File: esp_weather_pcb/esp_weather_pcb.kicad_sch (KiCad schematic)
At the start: 6 parts, among them U1 esp32_38P_Left, U2 esp32_38P_Right

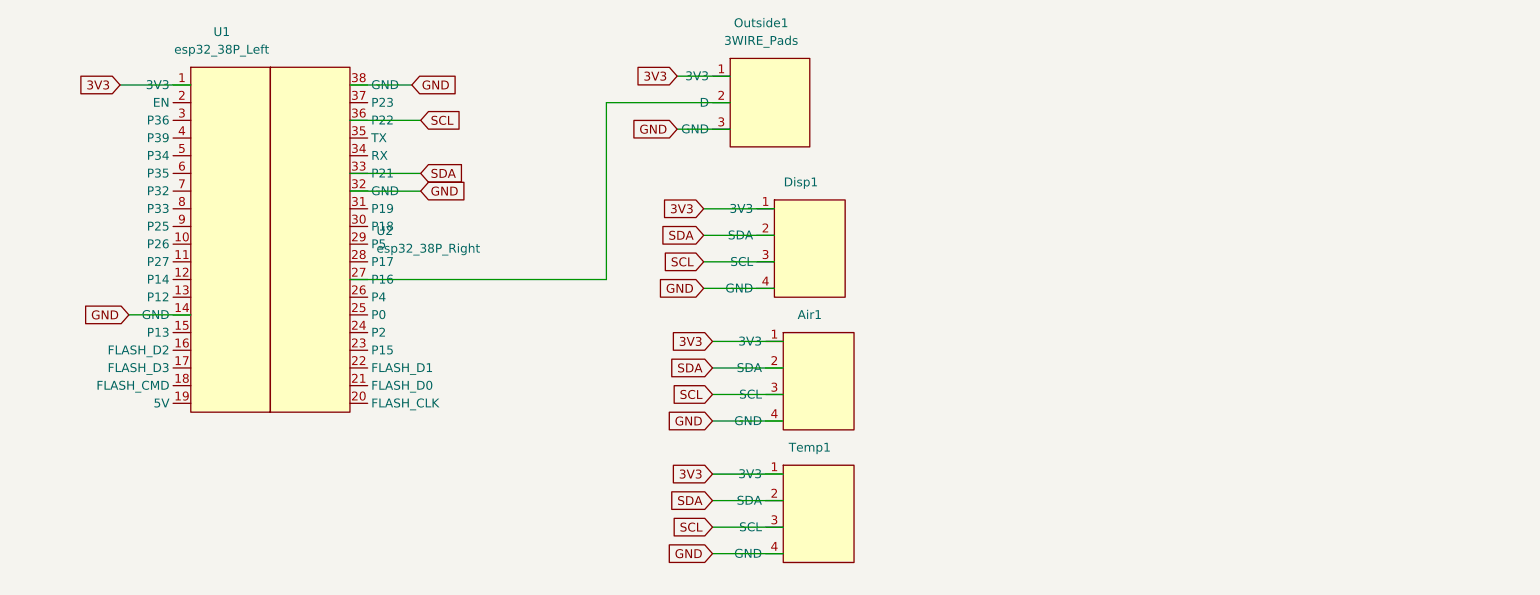
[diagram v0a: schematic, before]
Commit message: updated pcb
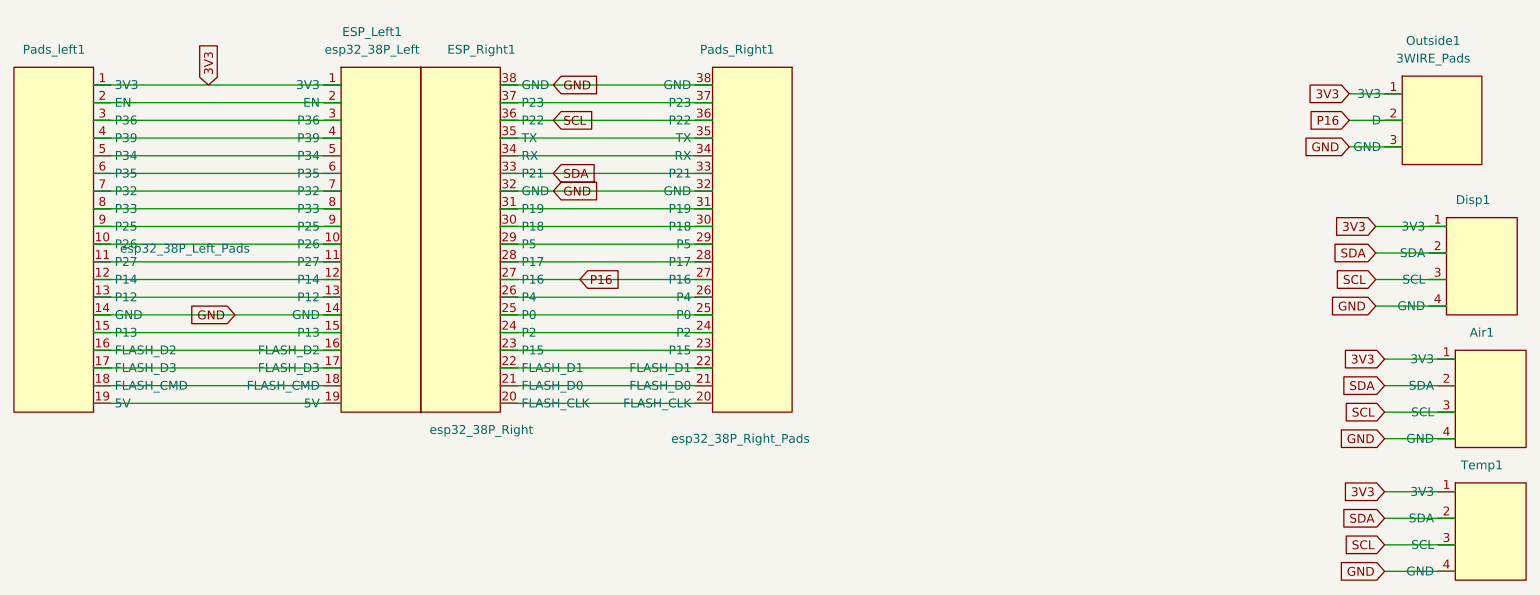
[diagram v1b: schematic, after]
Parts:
- added Pads_Right1: esp32_38P_Right_Pads, esp32_devboards:esp32_38P_right_pads, symbol esp32_devboards:esp32_38P_Right_Pads
- added Pads_left1: esp32_38P_Left_Pads, esp32_devboards:esp32_38P_left_Pads, symbol esp32_devboards:esp32_38P_Left_Pads
- renumbered U1 to ESP_Left1, U2 to ESP_Right1
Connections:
- net 3V3: now also Pads_left1.1 (3V3)
- net GND: now also Pads_Right1.32 (GND), Pads_Right1.38 (GND), Pads_left1.14 (GND)
- net SCL: now also Pads_Right1.36 (P22)
- net SDA: now also Pads_Right1.33 (P21)
- net at ESP_Right1.20 (FLASH_CLK): now also Pads_Right1.20 (FLASH_CLK)
- net at ESP_Right1.21 (FLASH_D0): now also Pads_Right1.21 (FLASH_D0)
- net at ESP_Right1.22 (FLASH_D1): now also Pads_Right1.22 (FLASH_D1)
- net at ESP_Right1.23 (P15): now also Pads_Right1.23 (P15)
- net at ESP_Right1.24 (P2): now also Pads_Right1.24 (P2)
- net at ESP_Right1.25 (P0): now also Pads_Right1.25 (P0)
- net at ESP_Right1.26 (P4): now also Pads_Right1.26 (P4)
- net P16: now reaches ESP_Right1.27 (P16), Outside1.2 (D)
- net P16: now also Pads_Right1.27 (P16)
- net at ESP_Right1.28 (P17): now also Pads_Right1.28 (P17)
- net at ESP_Right1.29 (P5): now also Pads_Right1.29 (P5)
- net at ESP_Right1.30 (P18): now also Pads_Right1.30 (P18)
- net at ESP_Right1.31 (P19): now also Pads_Right1.31 (P19)
- net at ESP_Right1.34 (RX): now also Pads_Right1.34 (RX)
- net at ESP_Right1.35 (TX): now also Pads_Right1.35 (TX)
- net at ESP_Right1.37 (P23): now also Pads_Right1.37 (P23)
- net at ESP_Left1.10 (P26): now also Pads_left1.10 (P26)
- net at ESP_Left1.11 (P27): now also Pads_left1.11 (P27)
- net at ESP_Left1.12 (P14): now also Pads_left1.12 (P14)
- net at ESP_Left1.13 (P12): now also Pads_left1.13 (P12)
- net at ESP_Left1.15 (P13): now also Pads_left1.15 (P13)
- net at ESP_Left1.16 (FLASH_D2): now also Pads_left1.16 (FLASH_D2)
- net at ESP_Left1.17 (FLASH_D3): now also Pads_left1.17 (FLASH_D3)
- net at ESP_Left1.18 (FLASH_CMD): now also Pads_left1.18 (FLASH_CMD)
- net at ESP_Left1.19 (5V): now also Pads_left1.19 (5V)
- net at ESP_Left1.2 (EN): now also Pads_left1.2 (EN)
- net at ESP_Left1.3 (P36): now also Pads_left1.3 (P36)
- net at ESP_Left1.4 (P39): now also Pads_left1.4 (P39)
- net at ESP_Left1.5 (P34): now also Pads_left1.5 (P34)
- net at ESP_Left1.6 (P35): now also Pads_left1.6 (P35)
- net at ESP_Left1.7 (P32): now also Pads_left1.7 (P32)
- net at ESP_Left1.8 (P33): now also Pads_left1.8 (P33)
- net at ESP_Left1.9 (P25): now also Pads_left1.9 (P25)
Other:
- moved on the sheet: Air1, Disp1, ESP_Left1, ESP_Right1, Outside1, Temp1
